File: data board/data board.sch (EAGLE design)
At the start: 43 parts, among them IC1 93LC56B, IC2 FT232HQ, U1 CJT1117-5.0-SOT223, X3 HUSB238, X6 USBC, Y1 12MHz

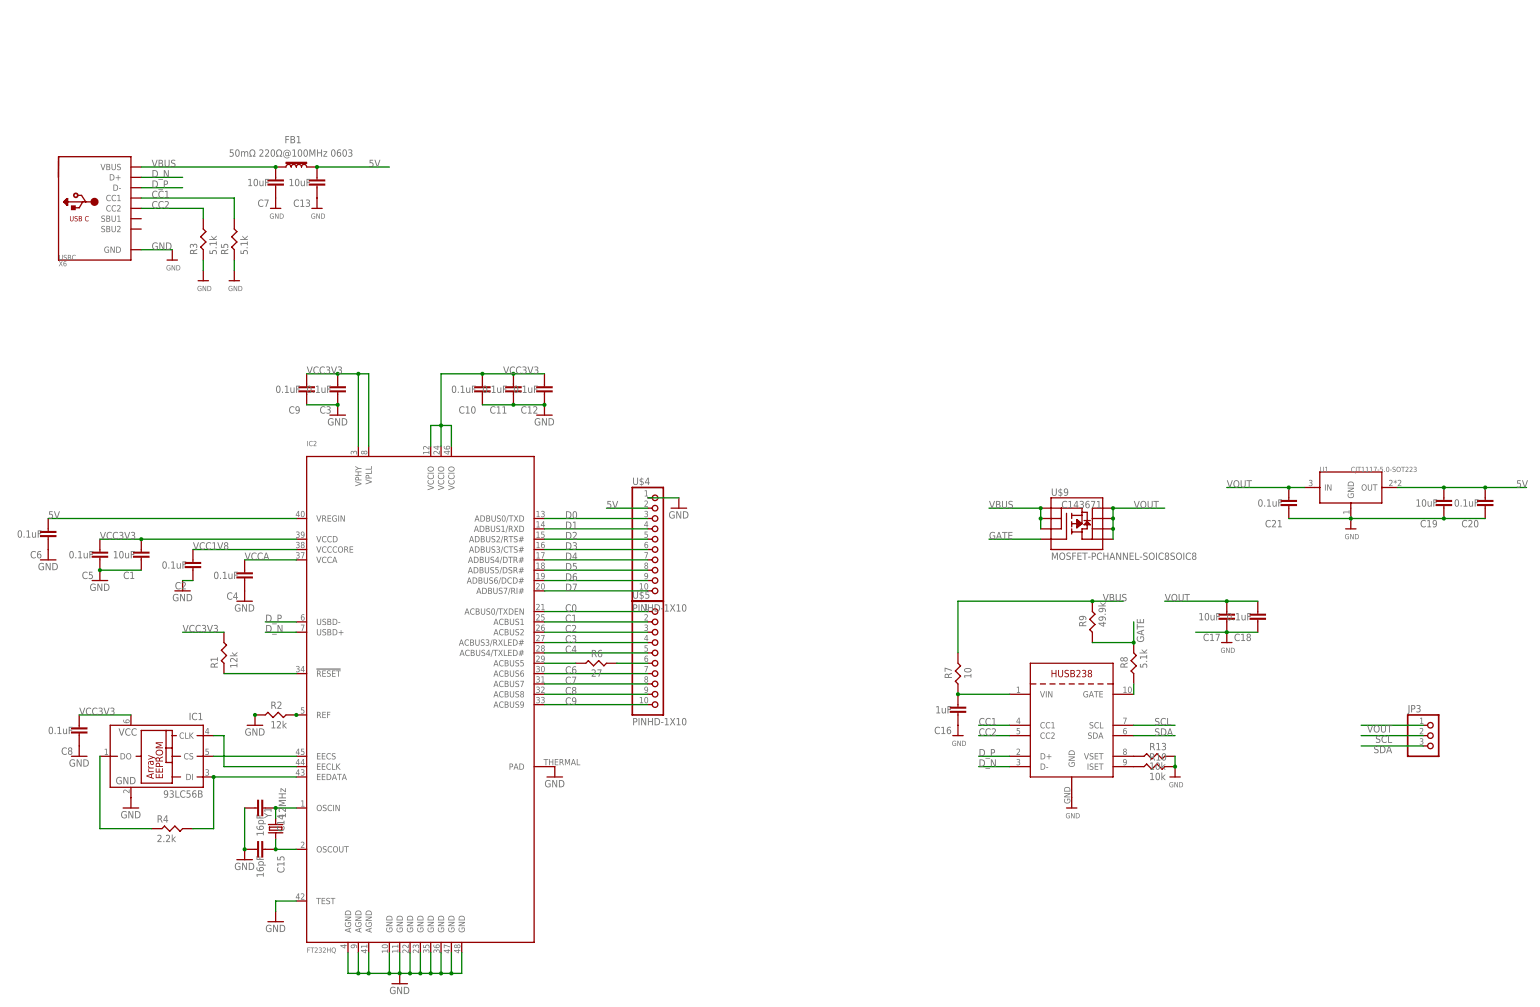
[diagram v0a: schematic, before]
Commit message: Revert "add husb238 for power delivery"
This reverts commit fdcc09ca80390afb5c840c7f1bf23dbb25893304.
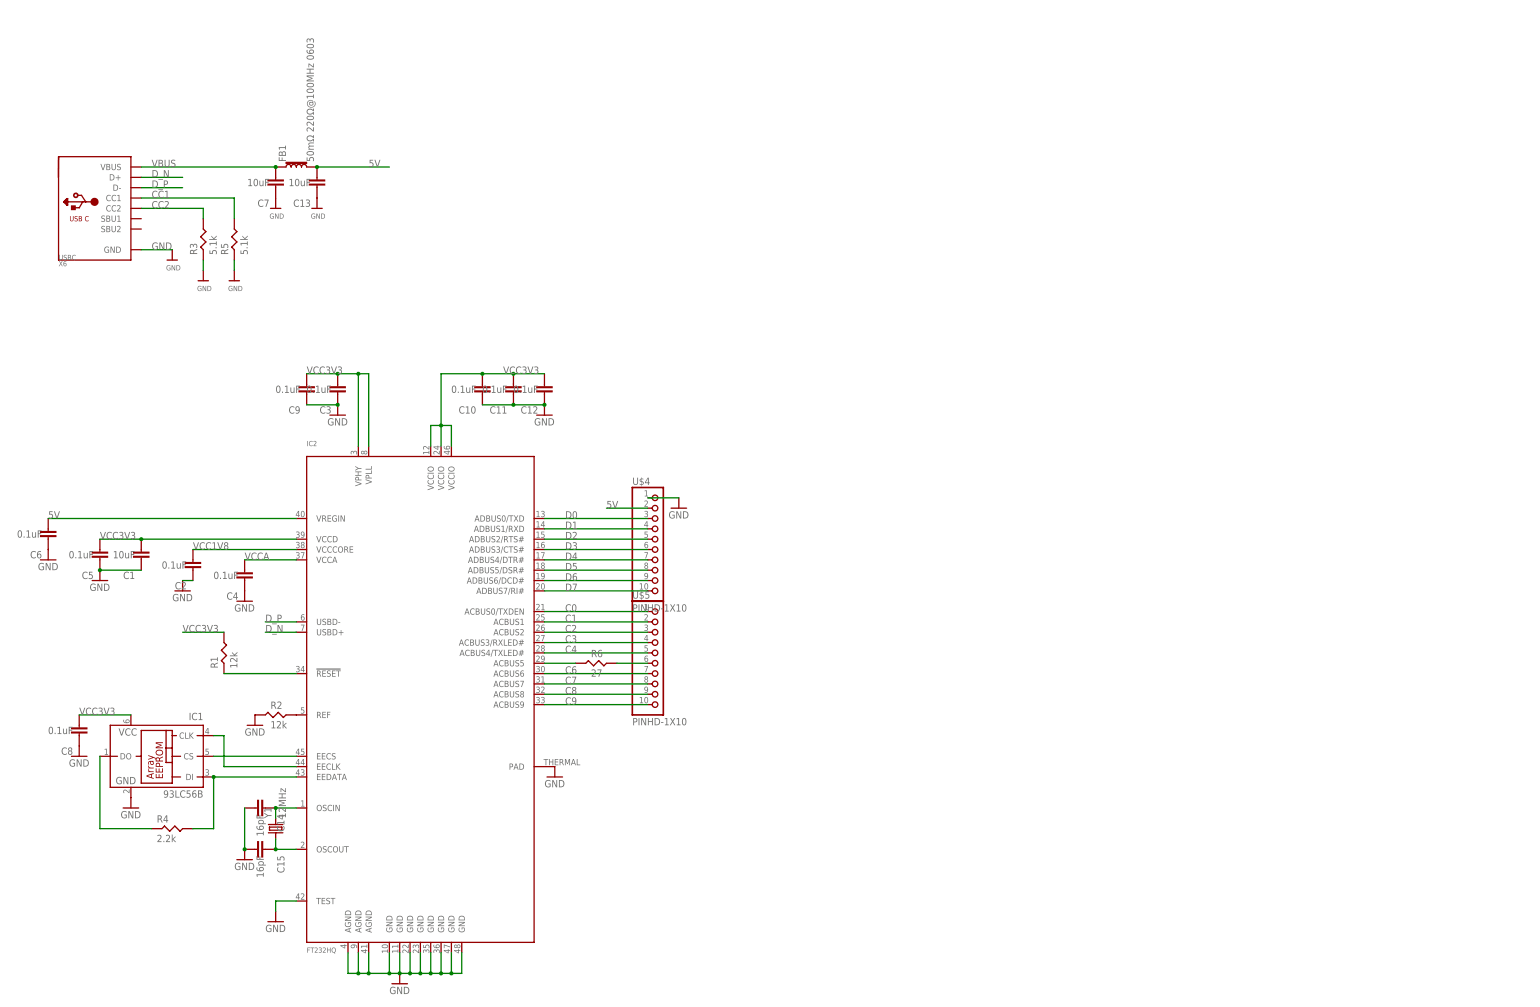
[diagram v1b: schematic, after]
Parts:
- removed C16: 1uF, Nordic_nRF:CAPACITOR_0402_N
- removed C17, C19: 10uF, Nordic_nRF:CAPACITOR_0805_N
- removed C18, C20, C21: 0.1uF, Nordic_nRF:CAPACITOR_0402_N
- removed JP3: (no value), microbuilder:HEADER-1X3ROUND
- removed R10, R13: 10k, FlashPCB_Resistors:RES-0402
- removed R7: 10, FlashPCB_Resistors:RES-0402
- removed R8: 5.1k, FlashPCB_Resistors:RES-0402
- removed R9: 49.9k, FlashPCB_Resistors:RES-0402
- removed U$9: MOSFET-PCHANNEL-SOIC8SOIC8, SparkFun-DiscreteSemi:MOSFET-PCHANNEL-SOIC8SOIC8
- removed U1: CJT1117-5.0-SOT223, Seeed-IC:PMIC-CJT1117-5.0(SOT223)
- removed X3: HUSB238, adafruit_power:HUSB238
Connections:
- removed net GATE: R8.P$2, R9.P$1, U$9.G
- removed net N$13: R13.P$1, X3.VSET
- removed net N$14: R10.P$1, X3.ISET
- removed net N$6: C16.2, R7.P$1, X3.VIN
- removed net N$8: R8.P$1, X3.GATE
- removed net SCL: JP3.2, X3.SCL
- removed net SDA: JP3.3, X3.SDA
- removed net VOUT: C17.2, C18.2, C21.2, JP3.1, U$9.D@1, U$9.D@2, U$9.D@3, U$9.D@4, U1.IN
- net 5V: no longer C19.2, C20.2, U1.OUT
- net CC1: no longer X3.CC1
- net CC2: no longer X3.CC2
- net D_N: no longer X3.D-
- net D_P: no longer X3.D+
- net GND: no longer C16.1, C17.1, C18.1, C19.1, C20.1, C21.1, R10.P$2, R13.P$2, U1.GND, X3.GND
- net VBUS: no longer R7.P$2, R9.P$2, U$9.S@1, U$9.S@2, U$9.S@3

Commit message: add husb238 for power delivery
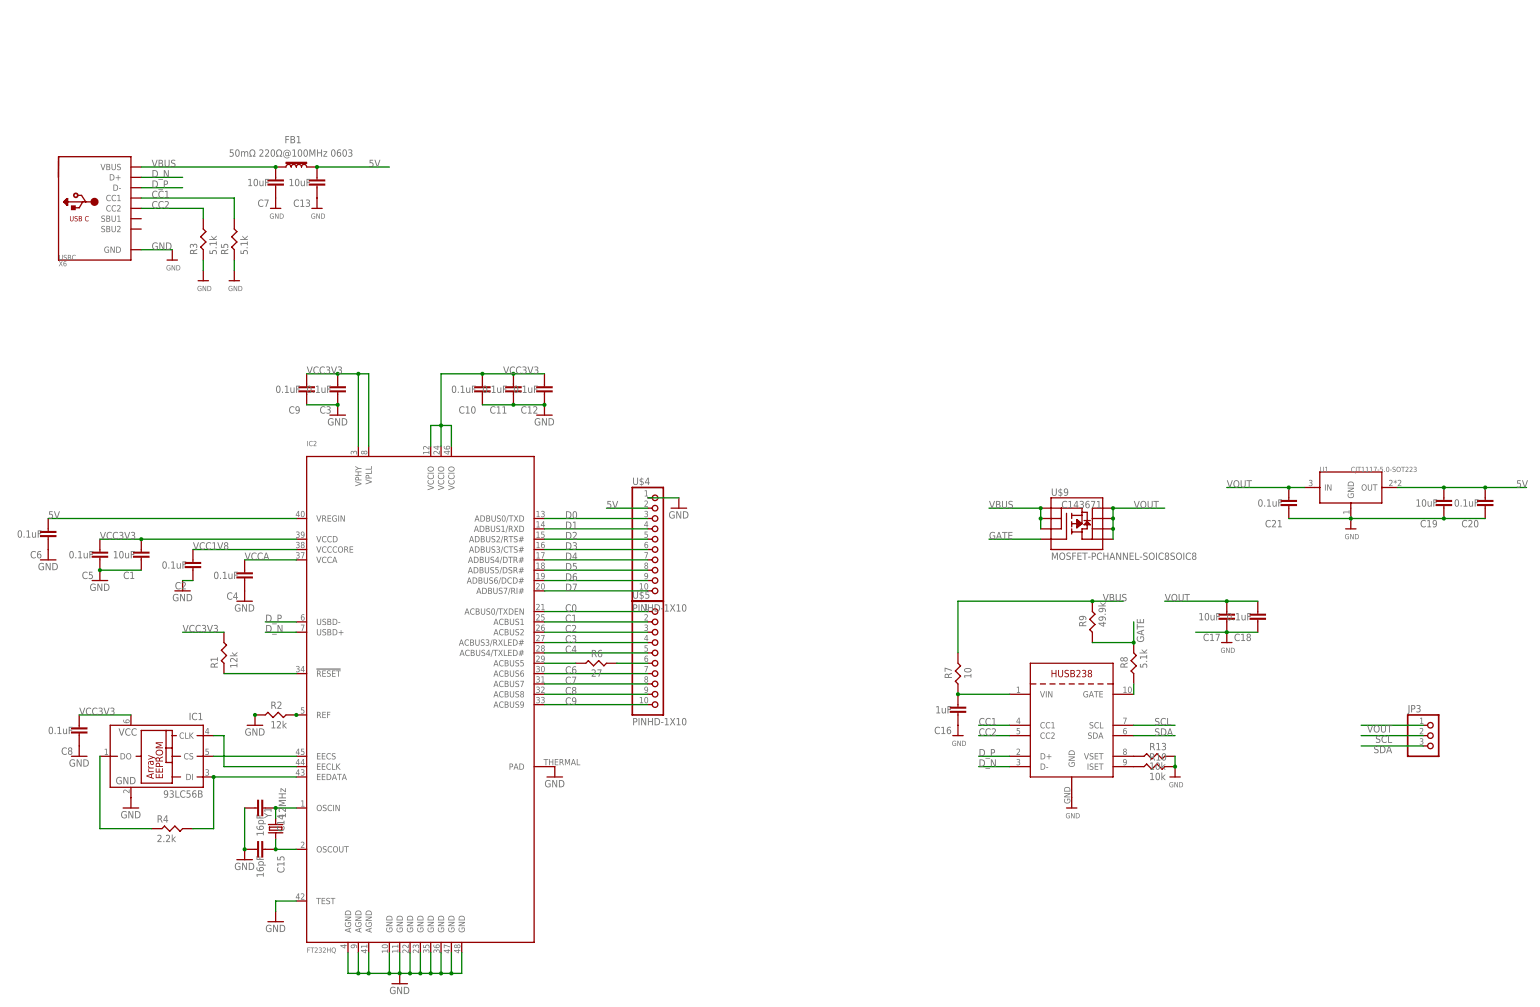
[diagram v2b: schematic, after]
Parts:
- added C16: 1uF, Nordic_nRF:CAPACITOR_0402_N
- added C17, C19: 10uF, Nordic_nRF:CAPACITOR_0805_N
- added C18, C20, C21: 0.1uF, Nordic_nRF:CAPACITOR_0402_N
- added JP3: (no value), microbuilder:HEADER-1X3ROUND
- added R10, R13: 10k, FlashPCB_Resistors:RES-0402
- added R7: 10, FlashPCB_Resistors:RES-0402
- added R8: 5.1k, FlashPCB_Resistors:RES-0402
- added R9: 49.9k, FlashPCB_Resistors:RES-0402
- added U$9: MOSFET-PCHANNEL-SOIC8SOIC8, SparkFun-DiscreteSemi:MOSFET-PCHANNEL-SOIC8SOIC8
- added U1: CJT1117-5.0-SOT223, Seeed-IC:PMIC-CJT1117-5.0(SOT223)
- added X3: HUSB238, adafruit_power:HUSB238
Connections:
- new net GATE: R8.P$2, R9.P$1, U$9.G
- new net N$13: R13.P$1, X3.VSET
- new net N$14: R10.P$1, X3.ISET
- new net N$6: C16.2, R7.P$1, X3.VIN
- new net N$8: R8.P$1, X3.GATE
- new net SCL: JP3.2, X3.SCL
- new net SDA: JP3.3, X3.SDA
- new net VOUT: C17.2, C18.2, C21.2, JP3.1, U$9.D@1, U$9.D@2, U$9.D@3, U$9.D@4, U1.IN
- net 5V: now also C19.2, C20.2, U1.OUT
- net CC1: now also X3.CC1
- net CC2: now also X3.CC2
- net D_N: now also X3.D-
- net D_P: now also X3.D+
- net GND: now also C16.1, C17.1, C18.1, C19.1, C20.1, C21.1, R10.P$2, R13.P$2, U1.GND, X3.GND
- net VBUS: now also R7.P$2, R9.P$2, U$9.S@1, U$9.S@2, U$9.S@3
